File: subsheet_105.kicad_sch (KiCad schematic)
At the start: 32 parts, among them SW2 RESET, U10 MC68000_DIP_64_PHY, U37 LM556_DUAL_TIMER_PHY

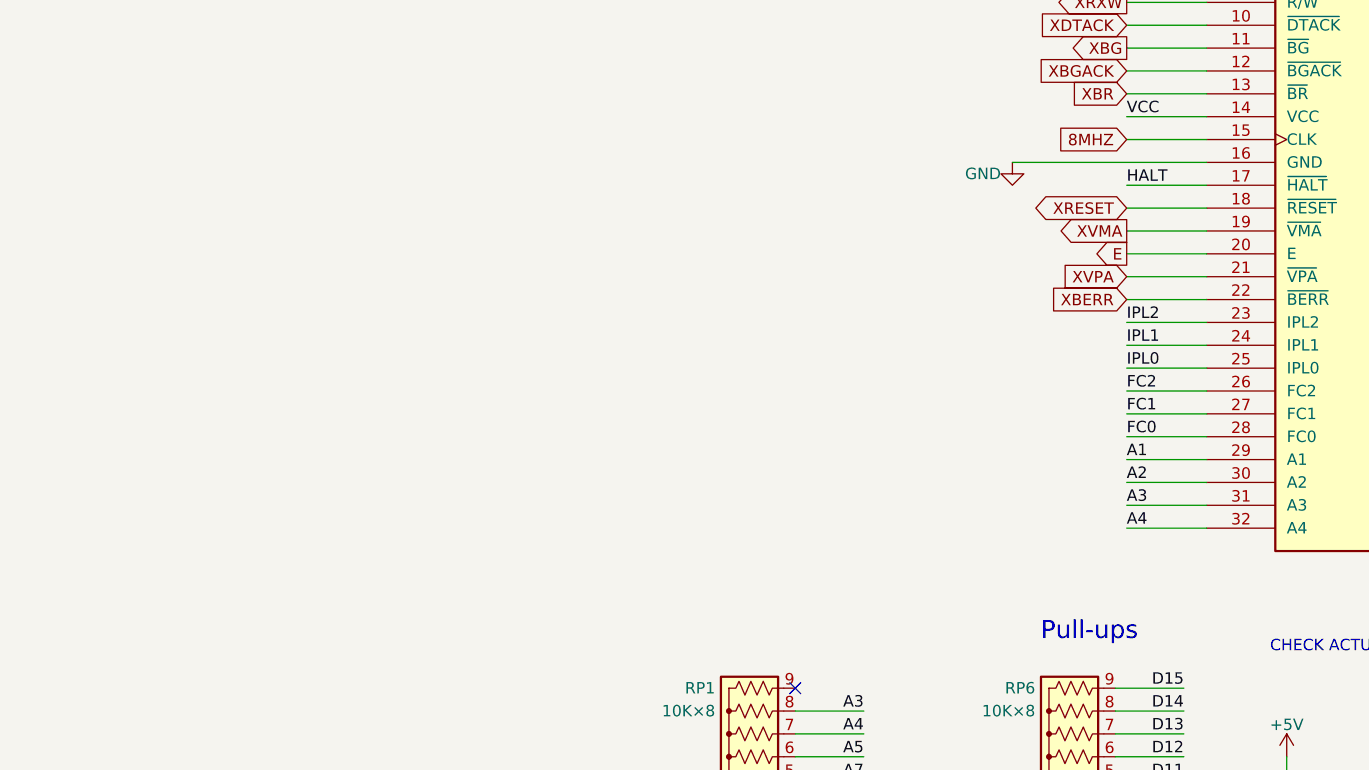
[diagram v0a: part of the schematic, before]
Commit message: finished reset circuit
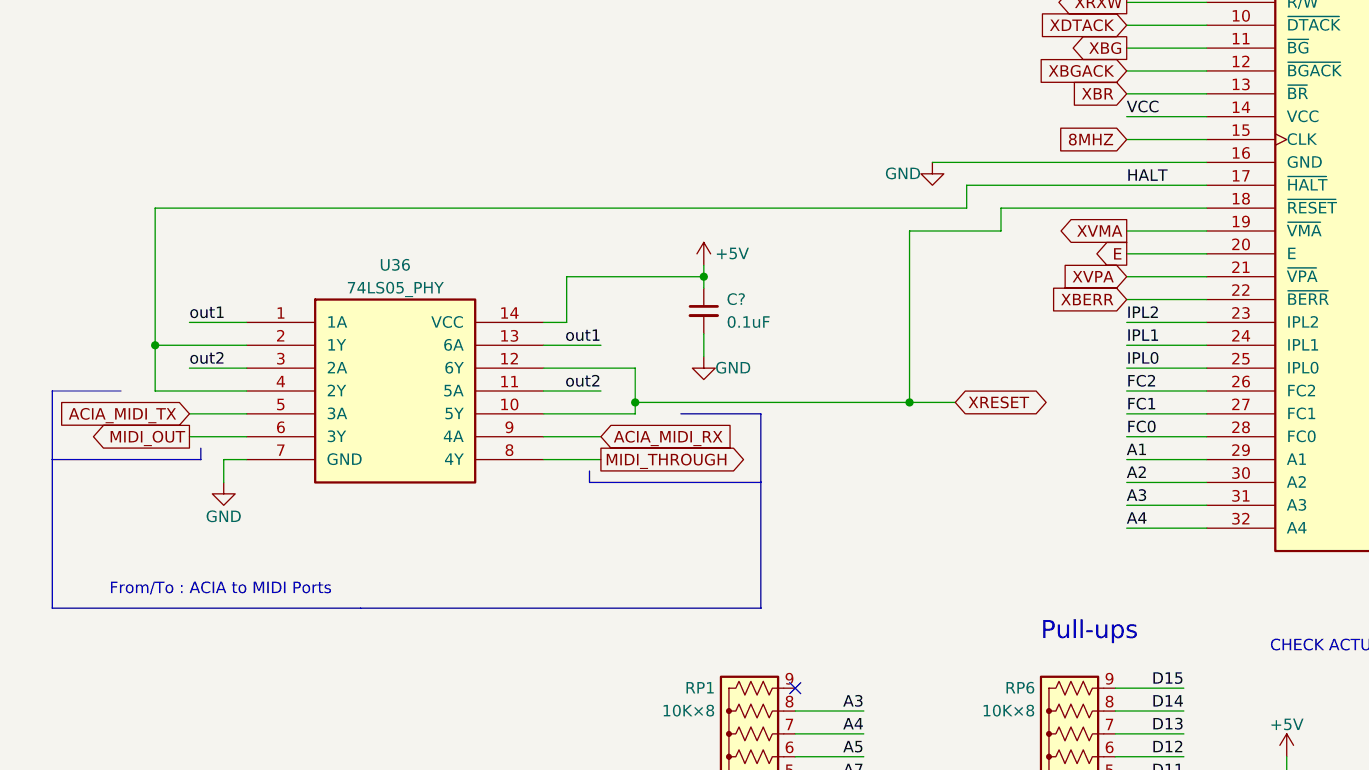
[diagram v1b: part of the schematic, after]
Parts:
- added C?: 0.1uF, commons-passives_THT:Passive_THT_capacitor_mlcc_W2.54mm_L12.70mm, symbol Device:C_Small
- added U36: 74LS05_PHY, Package_DIP:DIP-14_W7.62mm_LongPads, symbol 74x05:74LS05_PHY
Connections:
- net +5V: now also C?.1, U36.14 (VCC)
- net GND: now also C?.2, U36.7 (GND)
- net HALT: now also U36.2 (1Y), U36.4 (2Y)
- net XRESET: now also U36.10 (5Y), U36.12 (6Y)
- net out1: now also U36.1 (1A), U36.13 (6A)
- net out2: now also U36.11 (5A), U36.3 (2A)
- new net ACIA_MIDI_RX: U36.9 (4A)
- new net ACIA_MIDI_TX: U36.5 (3A)
- new net MIDI_OUT: U36.6 (3Y)
- new net MIDI_THROUGH: U36.8 (4Y)
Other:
- note added: "From/To : ACIA to MIDI Ports"
